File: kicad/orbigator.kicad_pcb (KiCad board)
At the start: 2 copper layers, 70 x 60 mm, 40 parts, among them J1 Conn_01x01, J10 Conn_01x01, J11 Conn_01x01, J12 Conn_01x01, J13 Conn_01x01, J14 Conn_01x01, J15 Conn_01x01, J16 Conn_01x01, J17 Conn_01x01, J18 Conn_01x01, J19 Conn_01x01, J2 Conn_01x01, J20 Conn_01x01, J21 Conn_01x01, J22 Conn_01x01, J23 Conn_01x01, J24 Conn_01x01, J25 Conn_01x01, J26 Conn_01x01, J27 Barrel_Jack_Switch, J28 Conn_01x01, J29 Conn_01x01, J3 Conn_01x01, J30 Conn_01x01, J4 Conn_01x01, J5 Conn_01x01, J6 Conn_01x01, J7 Conn_01x01, J8 Conn_01x01, J9 Conn_01x01, M1 DYNAMIXEL_1, M2 DYNAMIXEL_2, U1 Pico_2, U2 74LS126, U3 DC_polarity

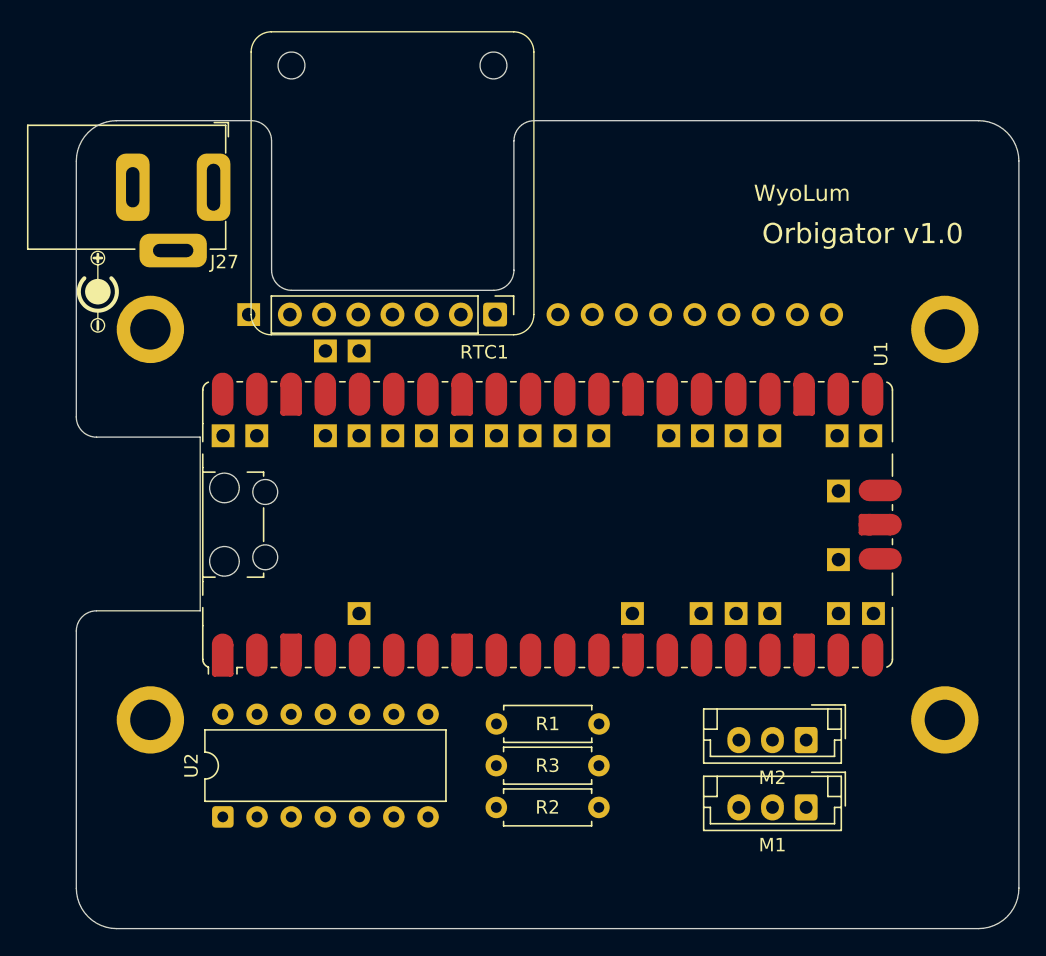
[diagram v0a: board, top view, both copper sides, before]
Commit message: PCB layout done
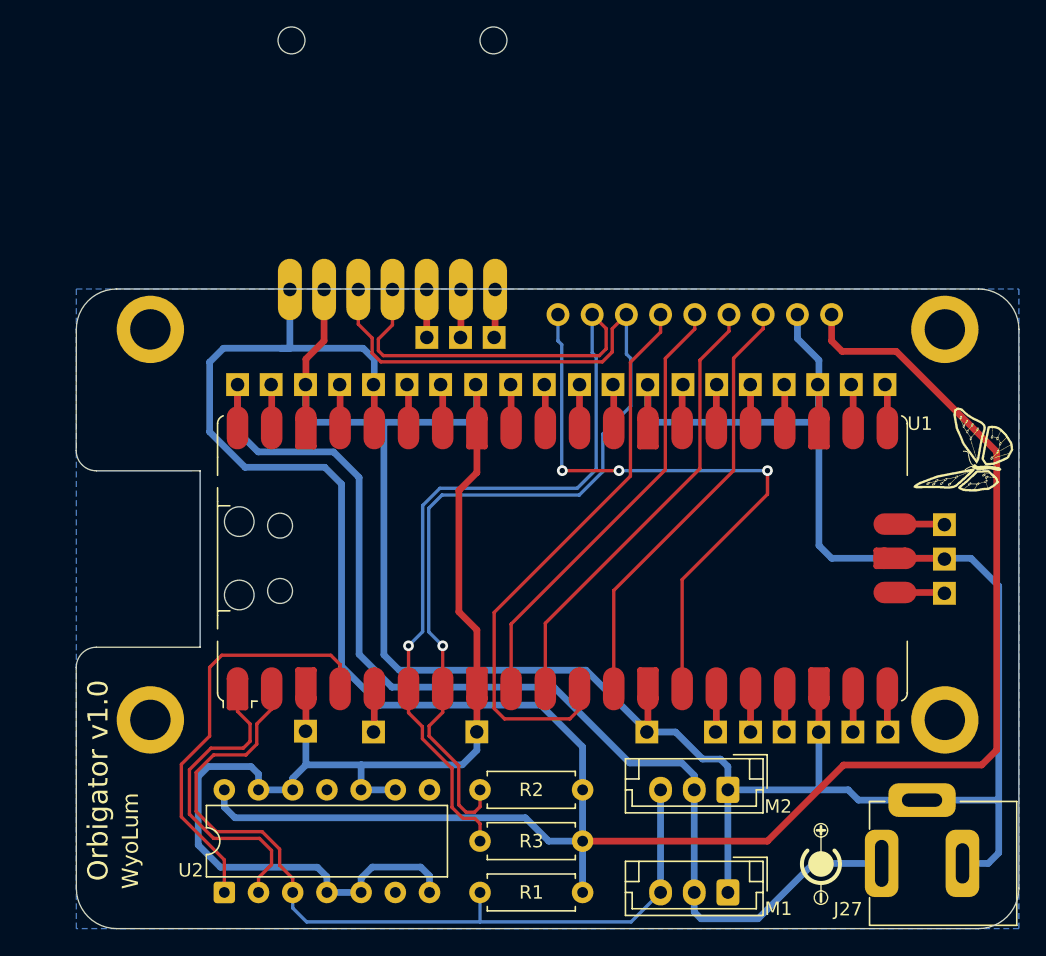
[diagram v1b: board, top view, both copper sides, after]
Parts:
- added G1: Logo-WL3, orbigator:logo-WL3, F.Cu at (124.6, 96.3)
- added J31: Conn_01x01, orbigator:PinHeader_1x01_P2.54mm_Vertical, F.Cu at (82.0, 115.3)
- added J32: Conn_01x01, orbigator:PinHeader_1x01_P2.54mm_Vertical, F.Cu at (129.5, 102.6)
- added J33: Conn_01x01, orbigator:PinHeader_1x01_P2.54mm_Vertical, F.Cu at (94.8, 115.4)
- added J34: Conn_01x01, orbigator:PinHeader_1x01_P2.54mm_Vertical, F.Cu at (82.0, 89.6)
- added J35: Conn_01x01, orbigator:PinHeader_1x01_P2.54mm_Vertical, F.Cu at (120.2, 115.4)
- added J36: Conn_01x01, orbigator:PinHeader_1x01_P2.54mm_Vertical, F.Cu at (120.1, 89.6)
- added J37: Conn_01x01, orbigator:PinHeader_1x01_P2.54mm_Vertical, F.Cu at (107.5, 89.6)
- RTC1: moved to B.Cu
- moved J27 70.6 mm to (124.8, 125.2), turned to 180 degrees
- moved U3 68.5 mm to (120.3, 125.2)
- moved J30 18.3 mm to (96.0, 86.1), turned to 180 degrees
- moved R1 12.6 mm to (102.6, 127.3)
- moved J29 10.0 mm to (93.5, 86.1), turned to 180 degrees
- moved J20 8.87 mm to (87.1, 115.4)
- moved J15 8.87 mm to (125.3, 115.4)
- moved J16 8.87 mm to (122.7, 115.4)
- moved J26 8.87 mm to (107.4, 115.4)
- moved J19 8.87 mm to (112.5, 115.4)
- moved J17 8.87 mm to (117.6, 115.4)
- moved J18 8.87 mm to (115.1, 115.4)
- moved M1 8.58 mm to (113.4, 127.3)
- moved R3 8.51 mm to (102.6, 123.5), turned to 180 degrees
- moved J21 8.29 mm to (129.5, 100.0)
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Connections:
- J12 pad 1: Net-(J12-Pin_1) -> /GND
- U1 pad 33: Net-(J12-Pin_1) -> /GND
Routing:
- net /GND: track 0.00 -> 289.2 mm
- net /3V3: track 0.00 -> 186.4 mm
- net /5V0: track 0.00 -> 84.9 mm
- net /SCL: track 0.00 -> 80.4 mm, vias 0 -> 1
- net /SDA: track 0.00 -> 78.8 mm, vias 0 -> 1
- net /MOT_DAT: track 0.00 -> 63.4 mm
- net /CNF_BTN: track 0.00 -> 45.8 mm, vias 0 -> 3
- net /ENC_SW: track 0.00 -> 42.8 mm
- net /ENC_B: track 0.00 -> 33.4 mm
- net /ENC_A: track 0.00 -> 33.4 mm
- net /BAK_BTN: track 0.00 -> 32.4 mm
- net /DIR: track 0.00 -> 31.1 mm
- net /UART_TX: track 0.00 -> 23.7 mm
- net Net-(J22-Pin_1): track 0.00 -> 4.47 mm
- net Net-(J21-Pin_1): track 0.00 -> 4.47 mm
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- added copper zone on B.Cu, net /GND
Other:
- board size 70 x 60 mm -> 70 x 47.5 mm
